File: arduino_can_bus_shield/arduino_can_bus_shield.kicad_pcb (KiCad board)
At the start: 2 copper layers, 68.6 x 53.3 mm, 8 parts, among them P1 Power, P2 Analog, P3 Digital, P4 Digital, P5 CONN_01X01, P6 CONN_01X01, P7 CONN_01X01, P8 CONN_01X01

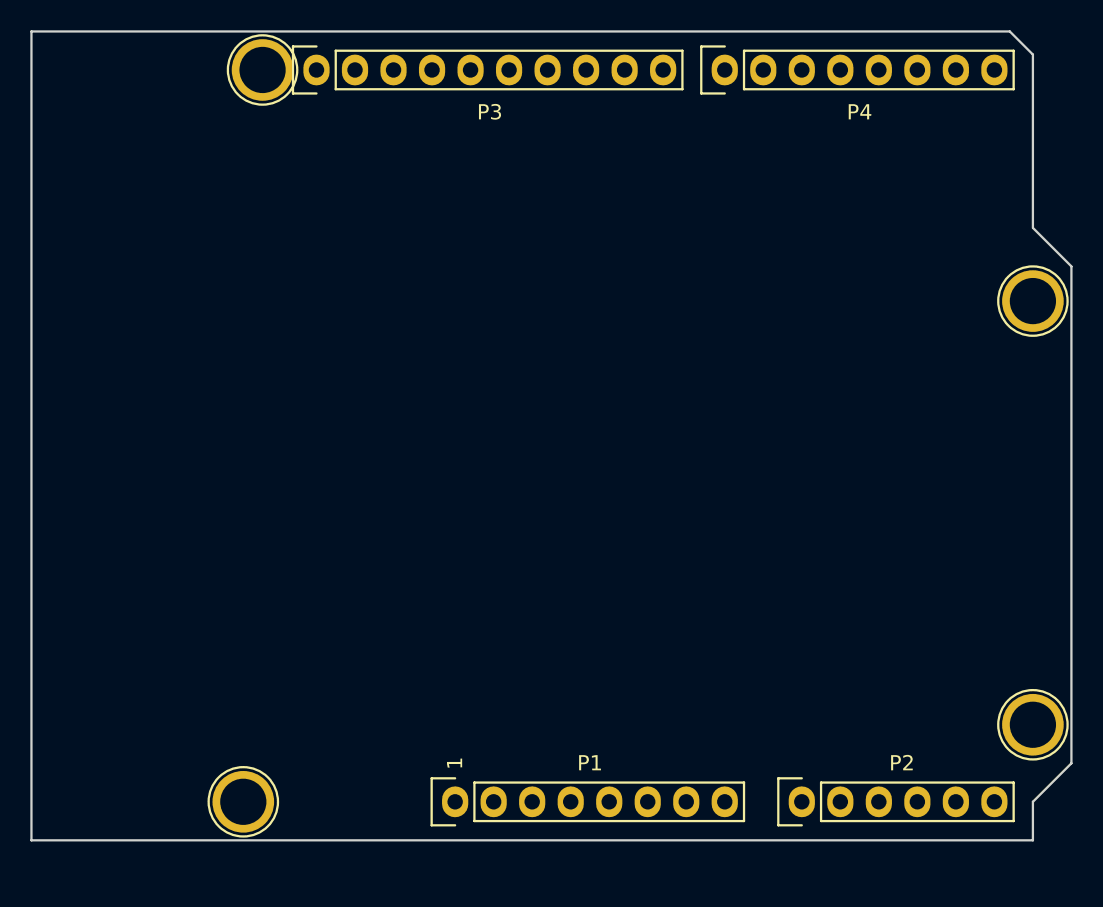
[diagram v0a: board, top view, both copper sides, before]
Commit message: ohh
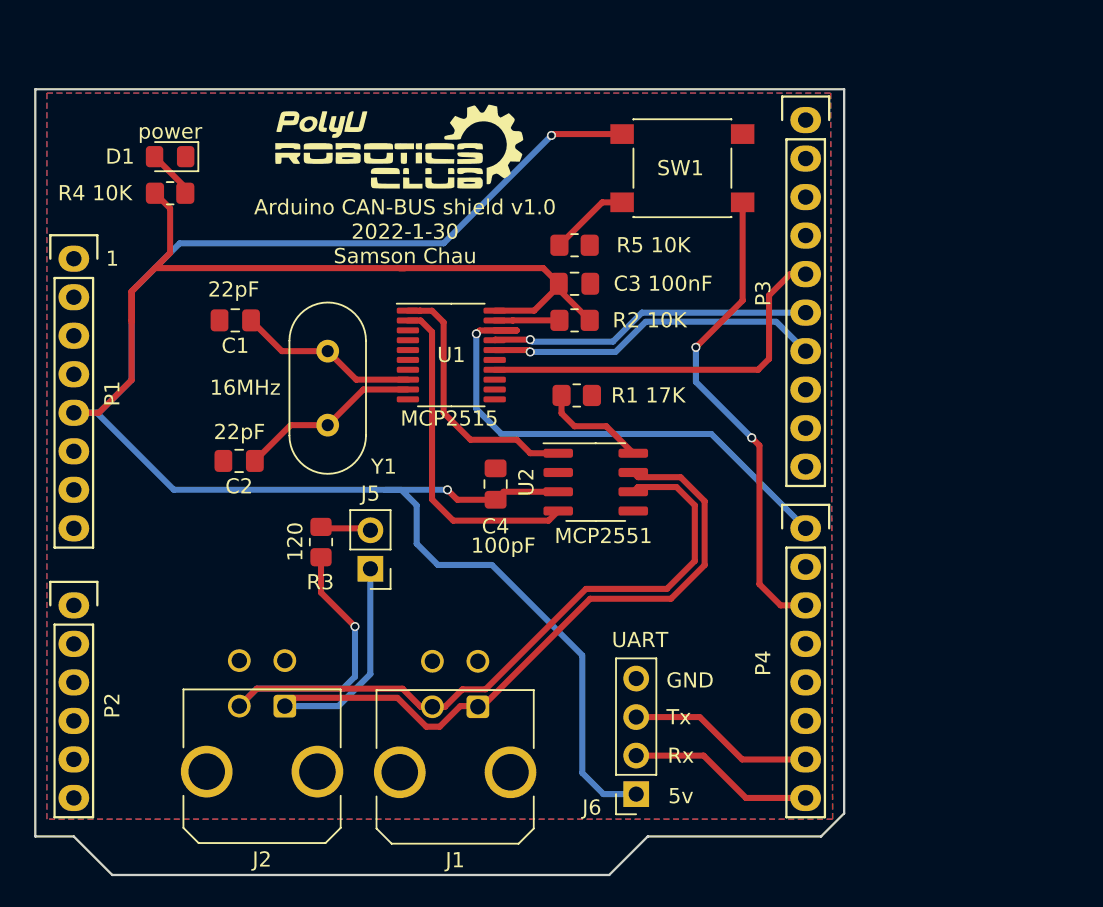
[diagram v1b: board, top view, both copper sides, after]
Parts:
- removed P5, P6, P7, P8: CONN_01X01, Socket_Arduino_Uno:Arduino_1pin
- added C1: 22pF, Capacitor_SMD:C_0805_2012Metric_Pad1.18x1.45mm_HandSolder, F.Cu at (124.4, 92.1)
- added C2: 22pF, Capacitor_SMD:C_0805_2012Metric_Pad1.18x1.45mm_HandSolder, F.Cu at (124.7, 101.3)
- added C3 100nF: 100nF, Capacitor_SMD:C_0805_2012Metric_Pad1.18x1.45mm_HandSolder, F.Cu at (146.8, 89.7)
- added C4: 100nF, Capacitor_SMD:C_0805_2012Metric_Pad1.18x1.45mm_HandSolder, F.Cu at (141.6, 102.9)
- added D1: power, LED_SMD:LED_0805_2012Metric_Pad1.15x1.40mm_HandSolder, F.Cu at (120.1, 81.3)
- added G***: LOGO, PolyuRobotics:Club_logo, F.Cu at (135.4, 80.9)
- added J1: molex_3.0, Connector_Molex:Molex_Micro-Fit_3.0_43045-0421_2x02-1MP_P3.00mm_Horizontal, F.Cu at (140.4, 117.6)
- added J2: molex_3.0, Connector_Molex:Molex_Micro-Fit_3.0_43045-0421_2x02-1MP_P3.00mm_Horizontal, F.Cu at (127.7, 117.5)
- added J5: jumper, Connector_PinHeader_2.54mm:PinHeader_1x02_P2.54mm_Vertical, F.Cu at (133.3, 108.5)
- added J6: UART2, Connector_PinSocket_2.54mm:PinSocket_1x04_P2.54mm_Vertical, F.Cu at (150.9, 123.3)
- added R1 17K: 17K, Resistor_SMD:R_0805_2012Metric_Pad1.20x1.40mm_HandSolder, F.Cu at (147.0, 97.0)
- added R2 10K: 10K, Resistor_SMD:R_0805_2012Metric_Pad1.20x1.40mm_HandSolder, F.Cu at (146.8, 92.1)
- added R3: 120, Resistor_SMD:R_0805_2012Metric_Pad1.20x1.40mm_HandSolder, F.Cu at (130.1, 106.7)
- added R4 10K: 10K, Resistor_SMD:R_0805_2012Metric_Pad1.20x1.40mm_HandSolder, F.Cu at (120.1, 83.7)
- added R5 10K: 10K, Resistor_SMD:R_0805_2012Metric_Pad1.20x1.40mm_HandSolder, F.Cu at (146.8, 87.1)
- added SW1: User, Button_Switch_SMD:SW_Push_1P1T_NO_6x6mm_H9.5mm, F.Cu at (153.9, 82.0)
- added U1: MCP2515-xST, Package_SO:TSSOP-20_4.4x6.5mm_P0.65mm, F.Cu at (138.7, 94.4)
- added U2: MCP2551-I-SN, Package_SO:SOIC-8_3.9x4.9mm_P1.27mm, F.Cu at (148.2, 102.7)
- added Y1: 16MHz, Crystal:Crystal_HC49-U_Vertical, F.Cu at (130.5, 94.1)
- moved P2 49.7 mm to (113.8, 110.9), turned to -90 degrees
- moved P1 43.8 mm to (113.8, 88.0), turned to -90 degrees
- moved P3 32.4 mm to (162.1, 78.9), turned to -90 degrees
- moved P4 30.7 mm to (162.1, 105.8), turned to -90 degrees
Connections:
- net /10(**/SS) renamed /10(**/SS)
- P1 pad 1: Net-(P1-Pad1) -> unconnected-(P1-Pad1)
- P3 pad 1: /A5(SCL) -> unconnected-(P3-Pad1)
- P3 pad 2: /A4(SDA) -> unconnected-(P3-Pad2)
- P3 pad 7: /11(**/MOSI) -> /11(**/MOSI)
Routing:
- net +5V: track 0.00 -> 169.2 mm, vias 0 -> 2
- net /CAN-: track 0.00 -> 60.6 mm, vias 0 -> 1
- net /CAN+: track 0.00 -> 56.3 mm
- net /5(**): track 0.00 -> 37.1 mm, vias 0 -> 2
- net /7: track 0.00 -> 34.1 mm, vias 0 -> 1
- net /13(SCK): track 0.00 -> 25.6 mm
- net /11(**/MOSI): track 0.00 -> 22.3 mm, vias 0 -> 1
- net /CAN_Rx: track 0.00 -> 22.1 mm
- net /12(MISO): track 0.00 -> 21.4 mm, vias 0 -> 1
- net /CAN_Tx: track 0.00 -> 17.3 mm
- net /1(Tx): track 0.00 -> 12.3 mm
- net /0(Rx): track 0.00 -> 12.3 mm
- net Net-(C2-Pad1): track 0.00 -> 12.0 mm
- net Net-(C1-Pad1): track 0.00 -> 12.0 mm
- net Net-(R1-Pad1): track 0.00 -> 7.00 mm
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- added copper zone on B.Cu, net GND
- added copper zone on F.Cu, net GND
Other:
- board size 68.6 x 53.3 mm -> 53.3 x 51.8 mm
- board text added: "100pF"
- board text added: "120"
- board text added: "16MHz"
- board text added: "22pF"
- board text added: "5v"
- board text added: "Arduino CAN-BUS shield v1.0 2022-1-30 Samson Chau"
- board text added: "GND"
- board text added: "MCP2515"
- board text added: "MCP2551"
- board text added: "Rx"
- board text added: "Tx"
- board text added: "UART"
- board text added: "power"
